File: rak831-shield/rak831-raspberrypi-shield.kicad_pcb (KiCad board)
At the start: 2 copper layers, 58.4 x 65.4 mm, 2 parts, among them P1 CONN_02X20, P2 CONN_02X12

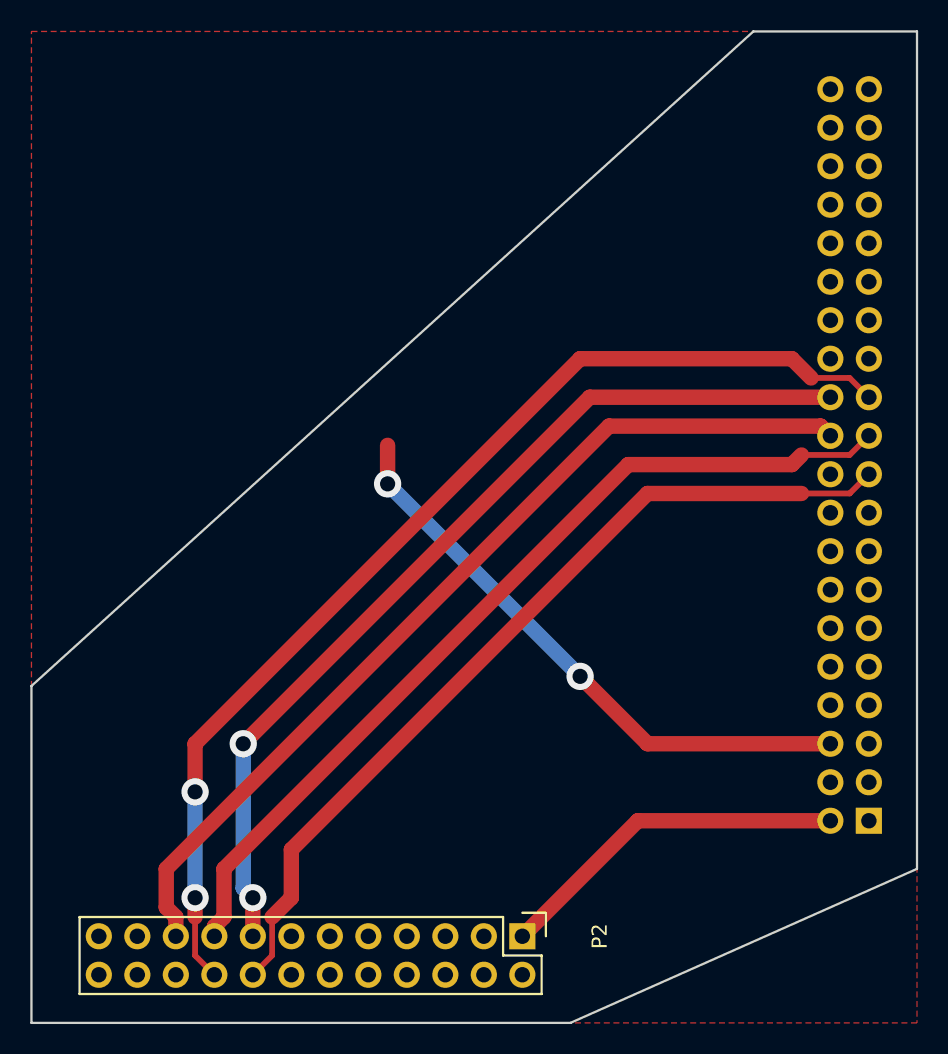
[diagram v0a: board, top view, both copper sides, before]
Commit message: Versión más compacta
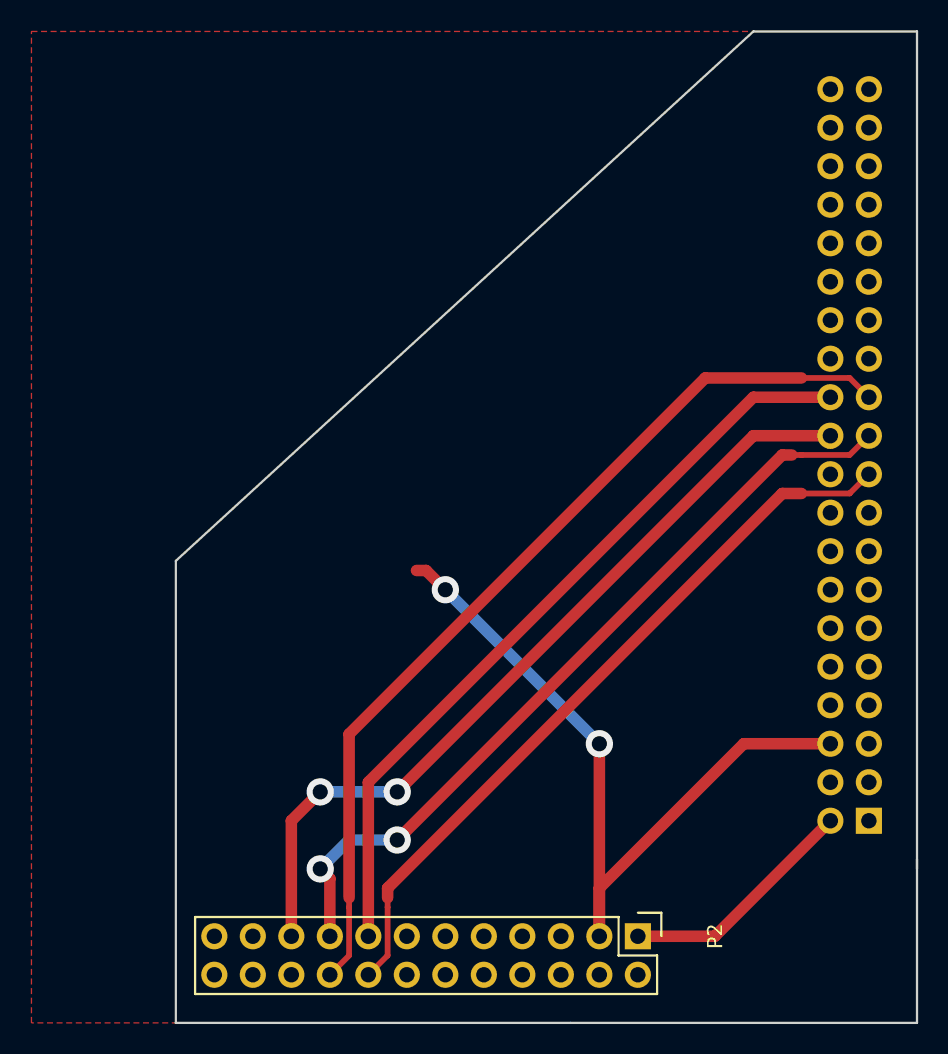
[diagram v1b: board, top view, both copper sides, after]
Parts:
- moved P2 7.62 mm to (119.4, 143.5)
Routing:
- net Net-(P1-Pad6): track 38.9 -> 51.9 mm
- net Net-(P1-Pad23): track 71.8 -> 61.6 mm, vias 2 -> 0
- net Net-(P1-Pad24): track 61.2 -> 51.2 mm, vias 2 -> 0
- net Net-(P1-Pad19): track 57.7 -> 49.9 mm
- net Net-(P1-Pad2): track 23.5 -> 15.9 mm
- net Net-(P1-Pad22): track 61.8 -> 54.6 mm, vias 0 -> 2
- net Net-(P1-Pad21): track 59.1 -> 52.7 mm, vias 0 -> 2
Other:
- board size 58.4 x 65.4 mm -> 48.9 x 65.4 mm
